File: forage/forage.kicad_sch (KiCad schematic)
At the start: 69 parts, among them J1 Conn_01x04_MountingPin, Q1 AO3400A, U1 STM32G431RBTx, U2 XC6206P322MR

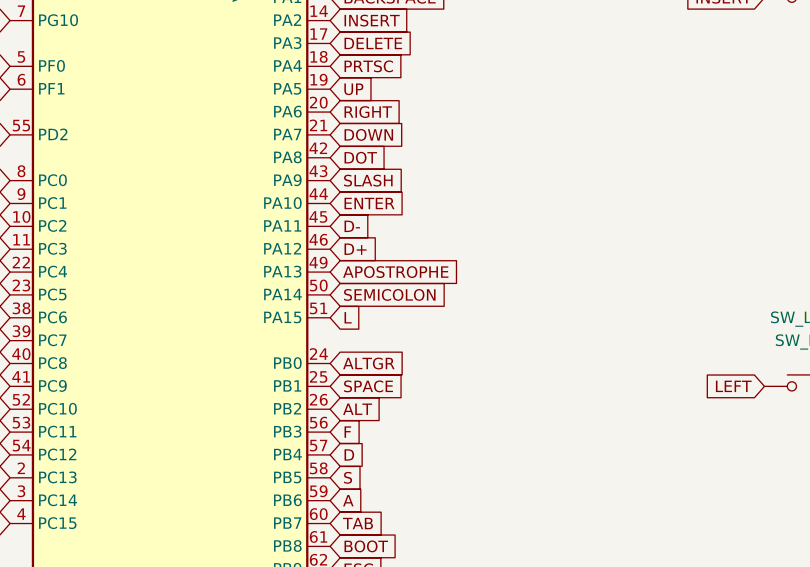
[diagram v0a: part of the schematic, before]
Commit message: wip: v2
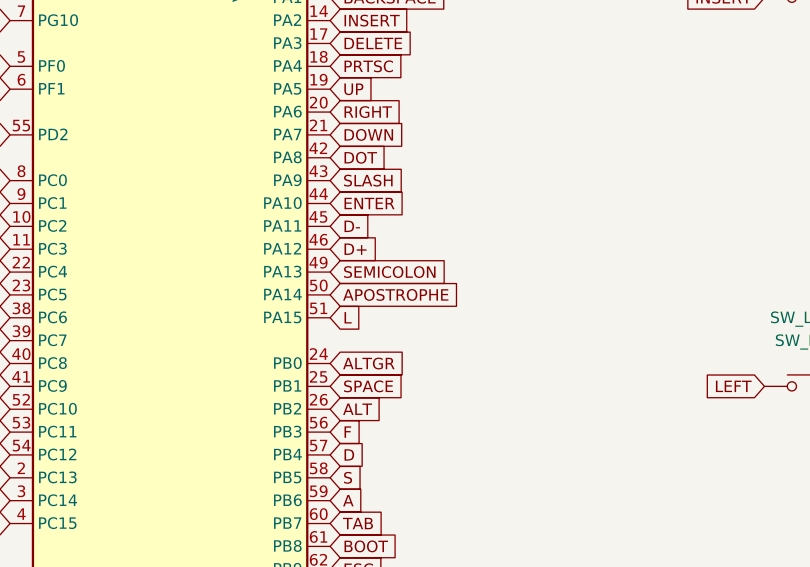
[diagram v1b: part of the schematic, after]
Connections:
- net APOSTROPHE: now also U1.50 (PA14); no longer U1.49 (PA13)
- net SEMICOLON: now also U1.49 (PA13); no longer U1.50 (PA14)
